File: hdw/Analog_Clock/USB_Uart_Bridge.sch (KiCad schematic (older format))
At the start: 31 parts

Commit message: a few sch adjustments
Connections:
- wire segments 57 -> 65
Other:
- note added: "ADD LEVEL SHIFTER/TRISTATE BUFFER STUFF"

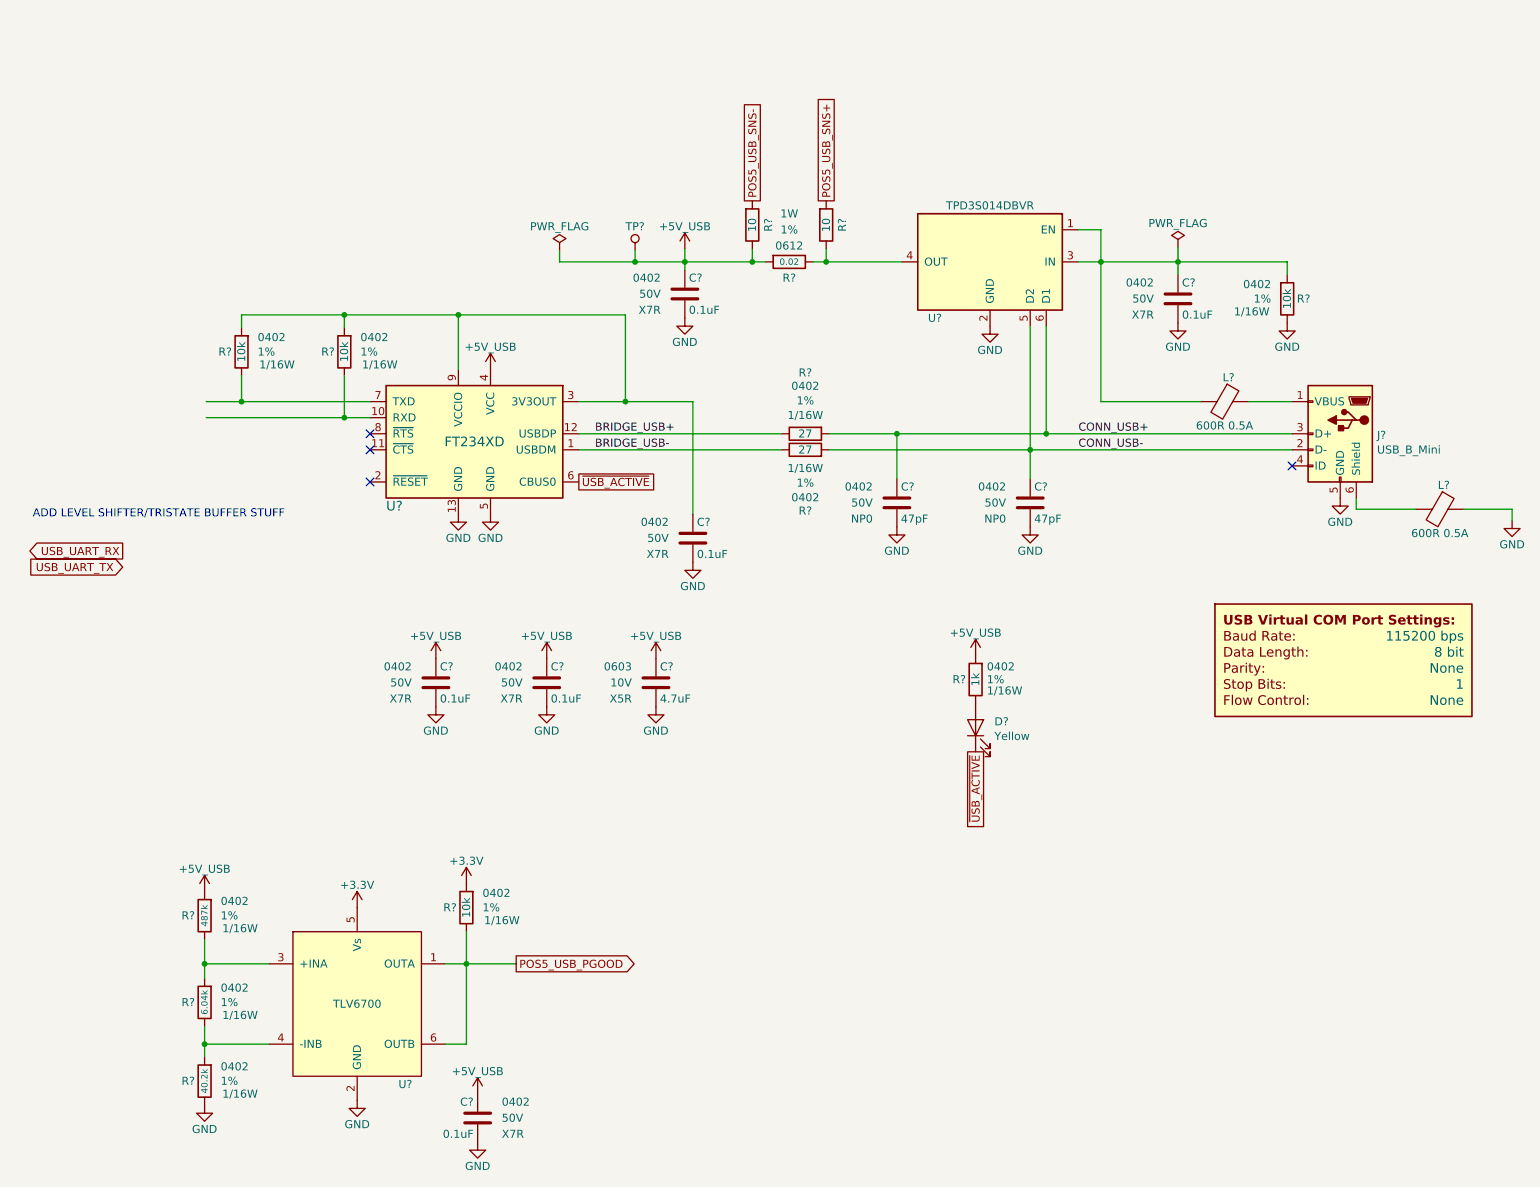
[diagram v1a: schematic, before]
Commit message: More sch work
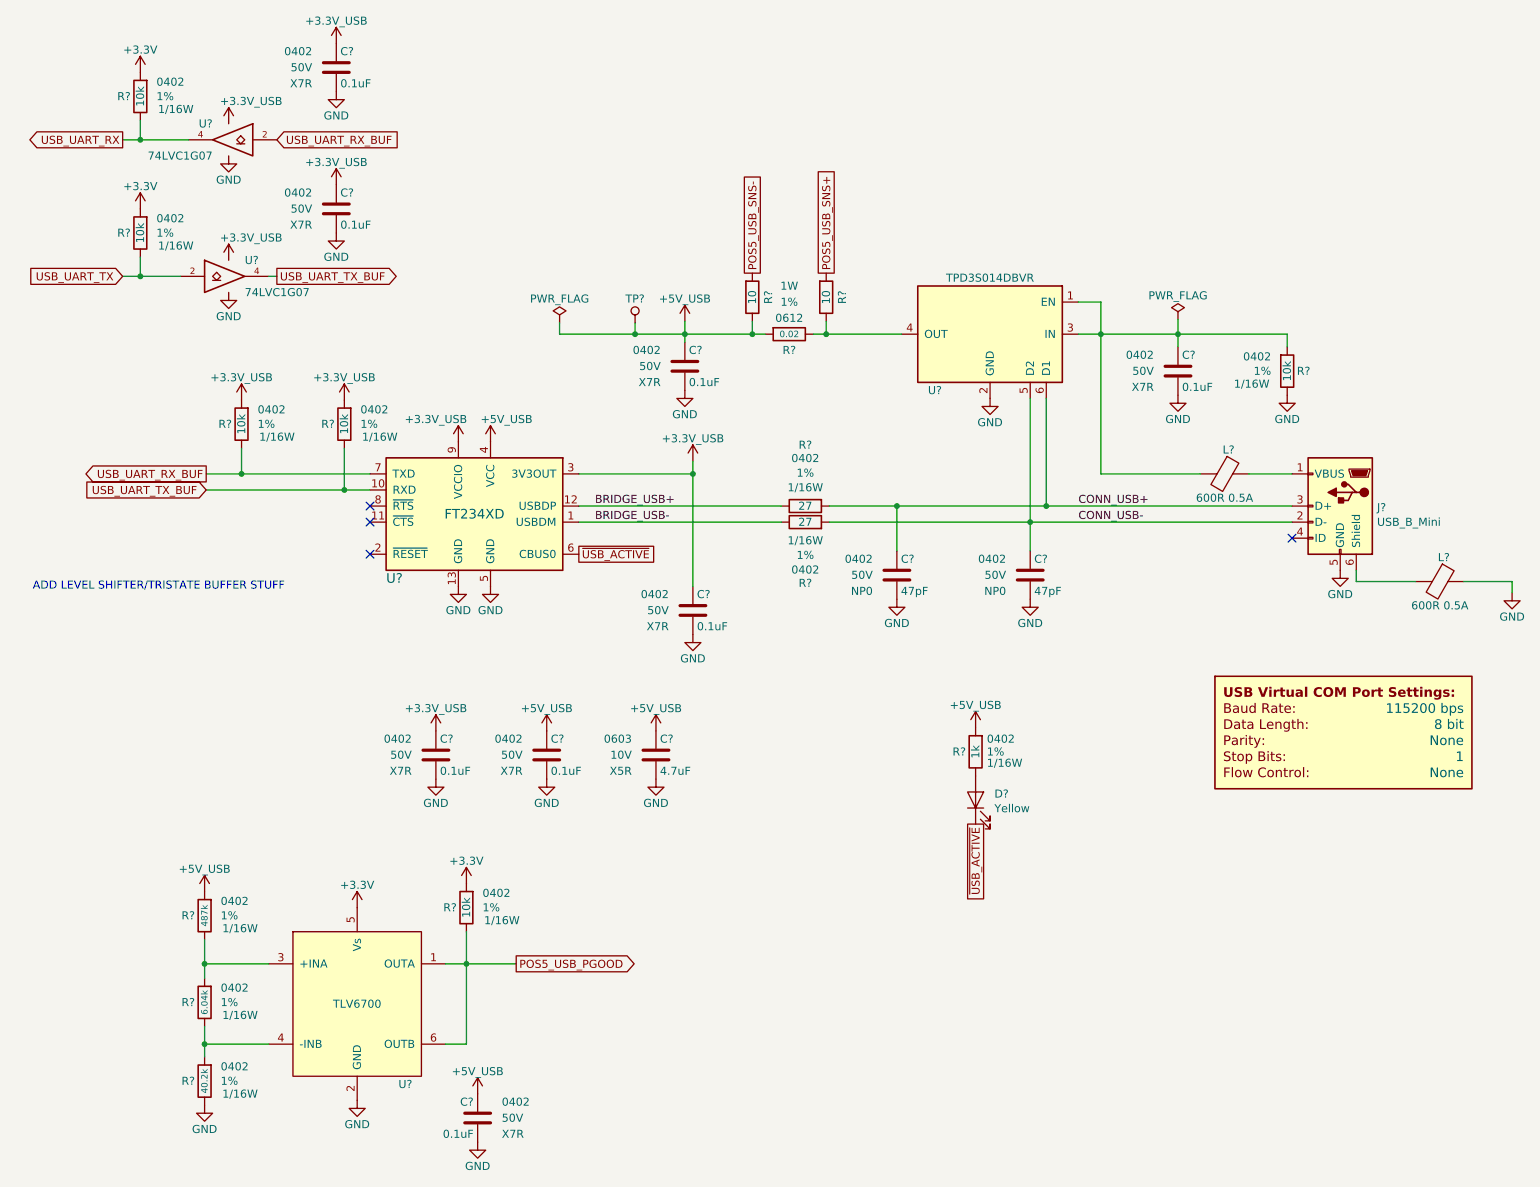
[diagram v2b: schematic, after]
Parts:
- added C? (x2): 0.1uF, Capacitors_SMD:C_0402, symbol Custom_Library:C_Custom
- added R? (x2): 10k, Resistors_SMD:R_0402, symbol Custom_Library:R_Custom
- added U? (x2): 74LVC1G07, TO_SOT_Packages_SMD:SOT-353_SC-70-5, symbol Custom_Library:74LVC1G07_Power
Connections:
- net labels added: +3.3V_USB, USB_UART_RX_BUF, USB_UART_TX_BUF
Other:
- moved on the sheet: C?, D?, J?, L?, R?, TP?, U?

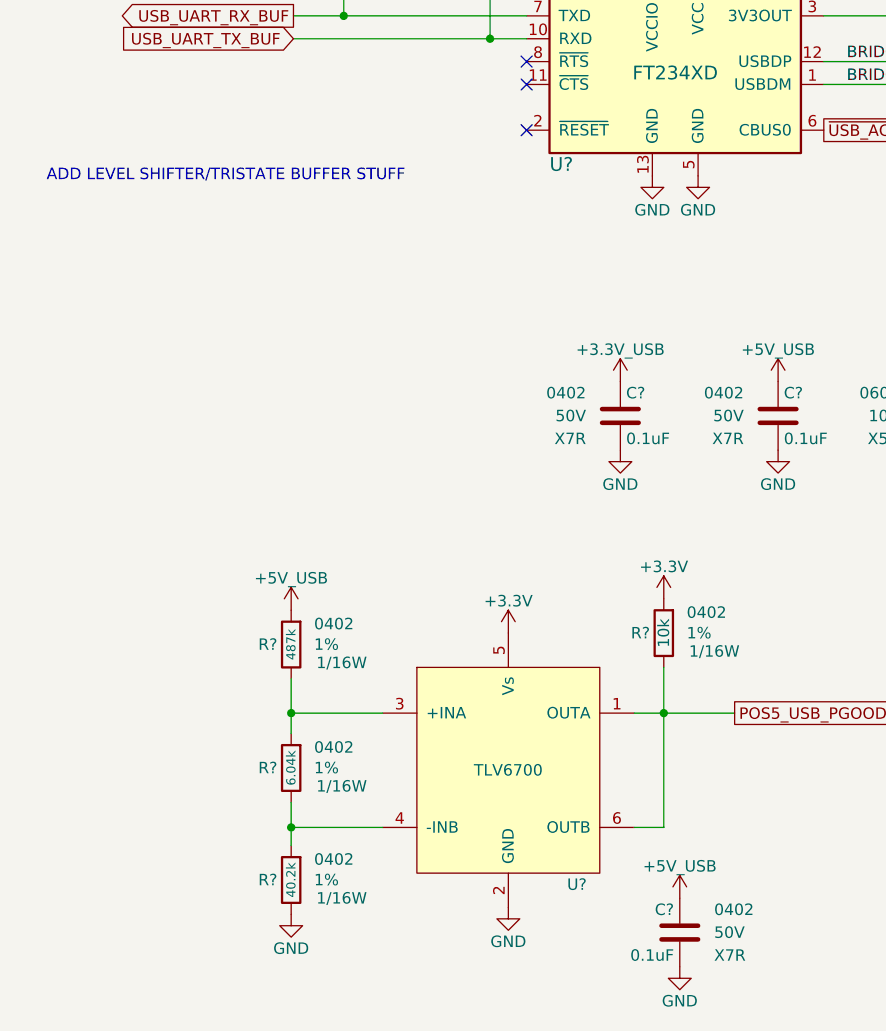
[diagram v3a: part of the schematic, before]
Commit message: more analog work, added some more sch stuff
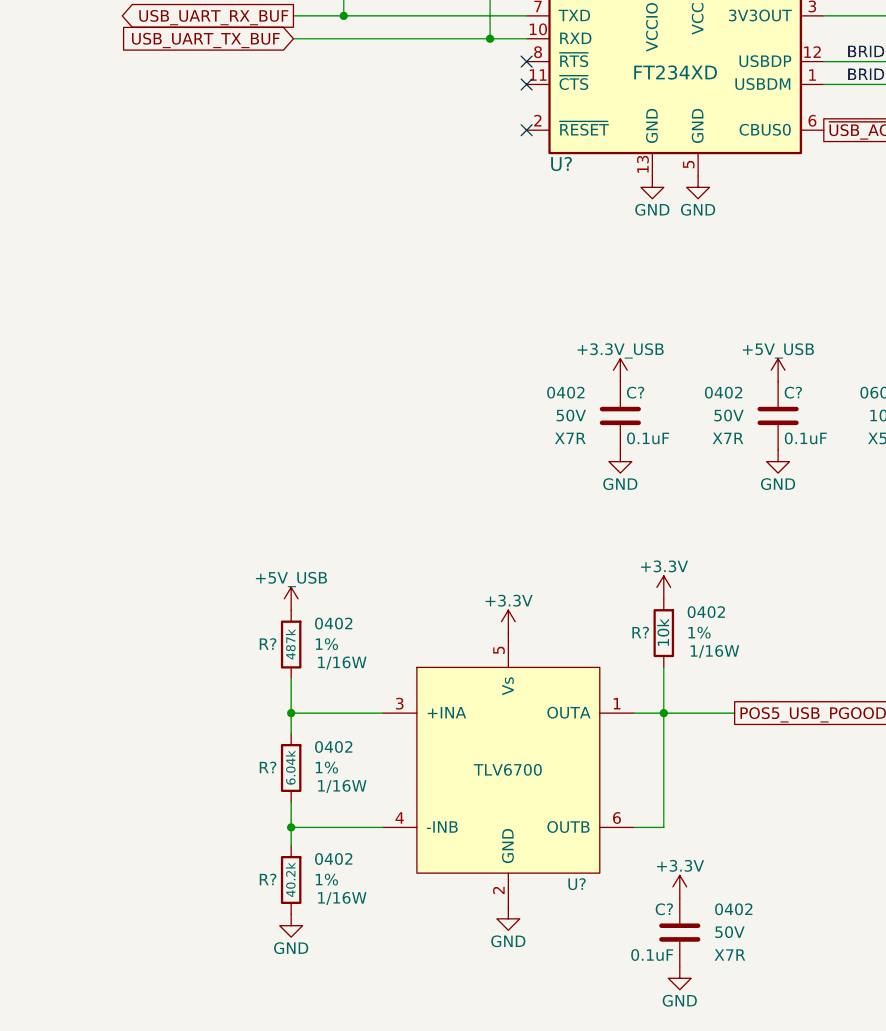
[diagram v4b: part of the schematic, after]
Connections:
- net +3V3: now also C?.1
- net +5V_USB: no longer C?.1
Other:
- note removed: "ADD LEVEL SHIFTER/TRISTATE BUFFER STUFF"
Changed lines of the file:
@@
 $Descr A 11000 8500
 encoding utf-8
-Sheet 13 23
+Sheet 13 24
 Title "VFD Clock"
 Date "2019-04-11"
@@
 	-1   0    0    -1
 $EndComp
-$Comp
-L Custom_Library:+5V_USB #PWR?
-U 1 1 5C037C4F
-P 3540 7400
-F 0 "#PWR?" H 3540 7250 50  0001 C CNN
-F 1 "+5V_USB" H 3540 7540 50  0000 C CNN
-F 2 "" H 3540 7400 50  0001 C CNN
-F 3 "" H 3540 7400 50  0001 C CNN
-	1    3540 7400
-	1    0    0    -1
-$EndComp
 Wire Wire Line
 	5730 3840 6980 3840
@@
 Wire Wire Line
 	8580 2670 7900 2670
-Text Notes 770  4270 0    50   ~ 0
-ADD LEVEL SHIFTER/TRISTATE BUFFER STUFF
 $Comp
 L power:GND #PWR?
@@
 	1    0    0    -1
 $EndComp
+$Comp
+L power:+3.3V #PWR?
+U 1 1 5F35E4BA
+P 3540 7400
+F 0 "#PWR?" H 3540 7250 50  0001 C CNN
+F 1 "+3.3V" H 3540 7540 50  0000 C CNN
+F 2 "" H 3540 7400 50  0001 C CNN
+F 3 "" H 3540 7400 50  0001 C CNN
+	1    3540 7400
+	1    0    0    -1
+$EndComp
